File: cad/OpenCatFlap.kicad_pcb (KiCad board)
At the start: 2 copper layers, 53.3 x 38.1 mm, 20 parts, among them P1 PIR Outside, P2 Flap IR Outside, P3 Flap IR Inside, P4 Servo Outside, P5 Servo Inside, P6 RFID Inside, P7 RFID Outside, P8 PIR Inside, U3 5V

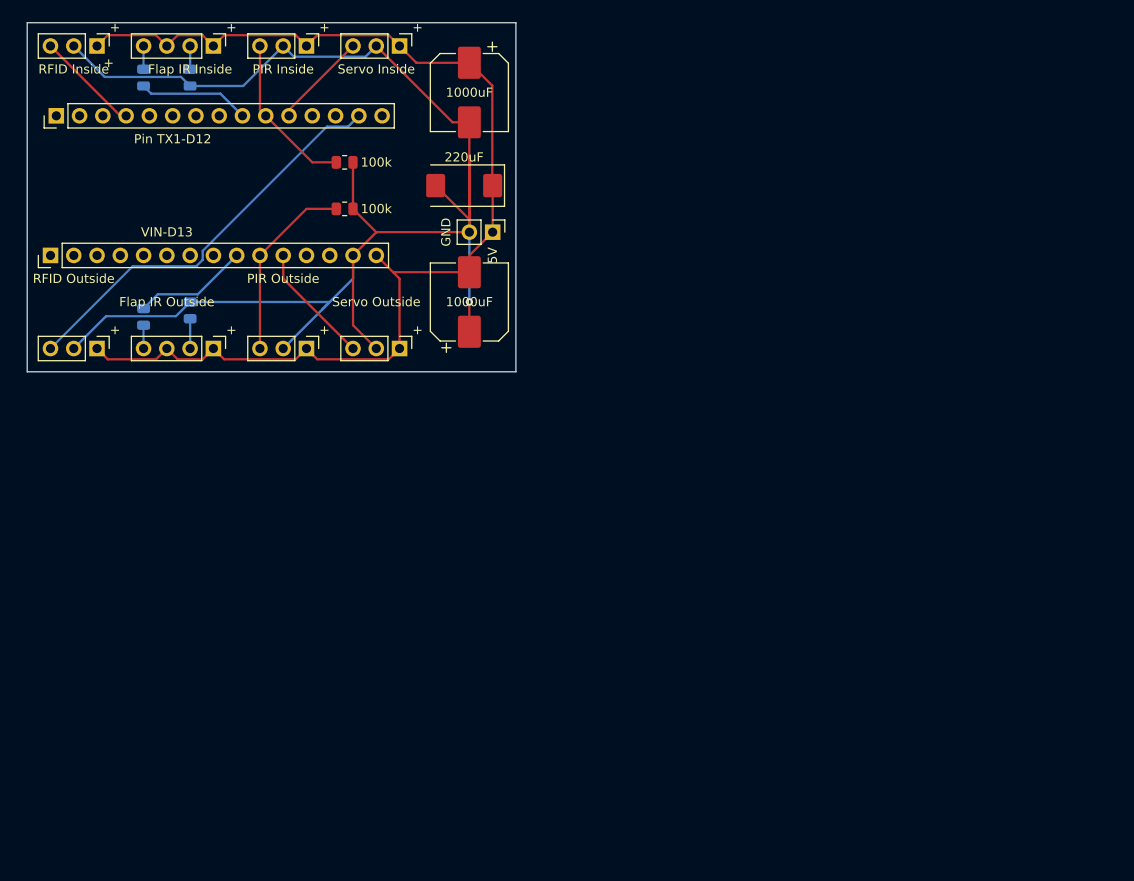
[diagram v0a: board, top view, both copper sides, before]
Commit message: v2§
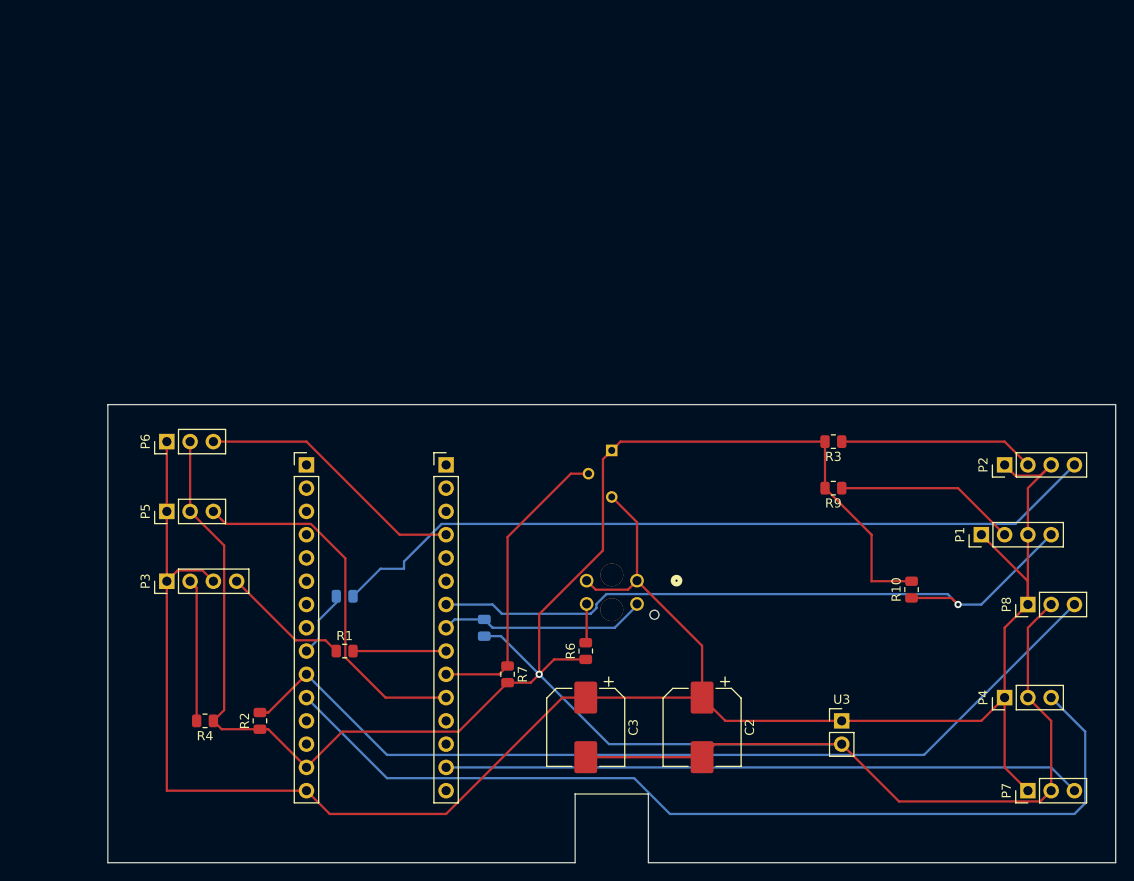
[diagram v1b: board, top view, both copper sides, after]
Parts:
- removed C4: 220uF, Capacitor_Tantalum_SMD:CP_EIA-7343-43_Kemet-X
- added PIR_IN1: AMN33111, OpenCatFlap:AMN33111_PAN, B.Cu at (155.0, 105.0)
- added R10: 10k, Resistor_SMD:R_0805_2012Metric, F.Cu at (187.7, 120.2)
- added R6: 200R, Resistor_SMD:R_0805_2012Metric, F.Cu at (152.2, 126.9)
- added R8: 10k, Resistor_SMD:R_0805_2012Metric, B.Cu at (141.1, 124.4)
- added R9: 200R, Resistor_SMD:R_0805_2012Metric, F.Cu at (179.2, 109.1)
- added U1: TCRT5000L, OpenCatFlap:TCRT5000_VIS, B.Cu at (157.8, 119.2)
- P1: value PIR Outside -> IR Outside; footprint Connector_PinHeader_2.54mm:PinHeader_1x03_P2.54mm_Vertical -> Connector_PinHeader_2.54mm:PinHeader_1x04_P2.54mm_Vertical
- P8: value PIR Inside -> PIR Outside
- R1, R3, R4: moved to F.Cu
- moved P7 112.5 mm to (200.4, 142.1), turned to 90 degrees
- moved P8 99.6 mm to (200.4, 121.8), turned to 90 degrees
- moved P2 87.3 mm to (197.9, 106.6), turned to 90 degrees
- moved P1 76.4 mm to (195.3, 114.2), turned to 90 degrees
- moved P4 76.2 mm to (197.9, 132.0), turned to 90 degrees
- moved C2 73.8 mm to (164.9, 135.2)
- moved R3 71.7 mm to (179.2, 104.0), turned to 180 degrees
- moved R4 70.2 mm to (110.6, 134.5), turned to 180 degrees
- moved R1 66.3 mm to (125.8, 126.9), turned to 0 degrees
- moved U3 65.5 mm to (180.1, 134.5), turned to 0 degrees
- moved P3 58.6 mm to (106.4, 119.3), turned to 90 degrees
- moved R7 58.6 mm to (143.6, 129.4), turned to -90 degrees
- moved ArduinoESP32_R1 57.1 mm to (136.9, 106.6), turned to 0 degrees
- moved P5 56.8 mm to (106.4, 111.7), turned to 90 degrees
- moved R2 56.6 mm to (116.6, 134.5), turned to 90 degrees
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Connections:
- ArduinoESP32_R1 pad 7: unconnected-(ArduinoESP32_R1-Pin_7-Pad7) -> Net-(ArduinoESP32_R1-Pin_7)
- ArduinoESP32_R1 pad 8: unconnected-(ArduinoESP32_R1-Pin_8-Pad8) -> Net-(ArduinoESP32_R1-Pin_8)
- C3 pad 1: Net-(ArduinoESP32_L1-Pin_14) -> Net-(ArduinoESP32_L1-Pin_15)
- C3 pad 2: Net-(ArduinoESP32_L1-Pin_15) -> Net-(ArduinoESP32_L1-Pin_14)
- P1 pad 2: Net-(ArduinoESP32_L1-Pin_14) -> Net-(P1-E-)
- P1 pad 3: Net-(ArduinoESP32_L1-Pin_10) -> Net-(ArduinoESP32_L1-Pin_15)
- P8 pad 3: Net-(ArduinoESP32_R1-Pin_10) -> Net-(ArduinoESP32_L1-Pin_10)
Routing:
- net Net-(ArduinoESP32_L1-Pin_14): track 167.1 -> 274.0 mm
- net Net-(ArduinoESP32_L1-Pin_15): track 126.7 -> 230.8 mm
- net Net-(ArduinoESP32_L1-Pin_11): track 13.3 -> 103.8 mm
- net Net-(P2-D-): track 2.54 -> 85.1 mm
- net Net-(ArduinoESP32_L1-Pin_10): track 20.6 -> 101.1 mm
- net Net-(ArduinoESP32_R1-Pin_7): track 0.00 -> 76.6 mm, vias 0 -> 1
- net Net-(ArduinoESP32_R1-Pin_11): track 10.5 -> 40.2 mm
- net Net-(ArduinoESP32_R1-Pin_14): track 44.7 -> 69.6 mm
- net Net-(ArduinoESP32_R1-Pin_8): track 0.00 -> 22.8 mm
- net Net-(P1-E-): track 0.00 -> 19.9 mm
- net Net-(P2-E-): track 3.25 -> 21.4 mm
- net Net-(ArduinoESP32_R1-Pin_4): track 12.0 -> 29.6 mm
- net Net-(ArduinoESP32_R1-Pin_10): track 17.7 -> 32.9 mm
- net Net-(P3-E-): track 2.54 -> 15.5 mm
- net Net-(P3-D-): track 2.54 -> 14.0 mm
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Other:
- board size 53.3 x 38.1 mm -> 110 x 50 mm
- board text removed: "+"
- board text removed: "1000uF"
- board text removed: "GND"
